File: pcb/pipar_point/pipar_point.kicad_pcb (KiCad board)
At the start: 2 copper layers, 145.3 x 110.3 mm, 118 parts, among them Q1 AO3416 N-channel MOSFET, SW1 SW_Wuerth_450301014042, SW2 CK_KMS2xxG, U1 Seeeduino Xiao nRF52840, U2 74HC595

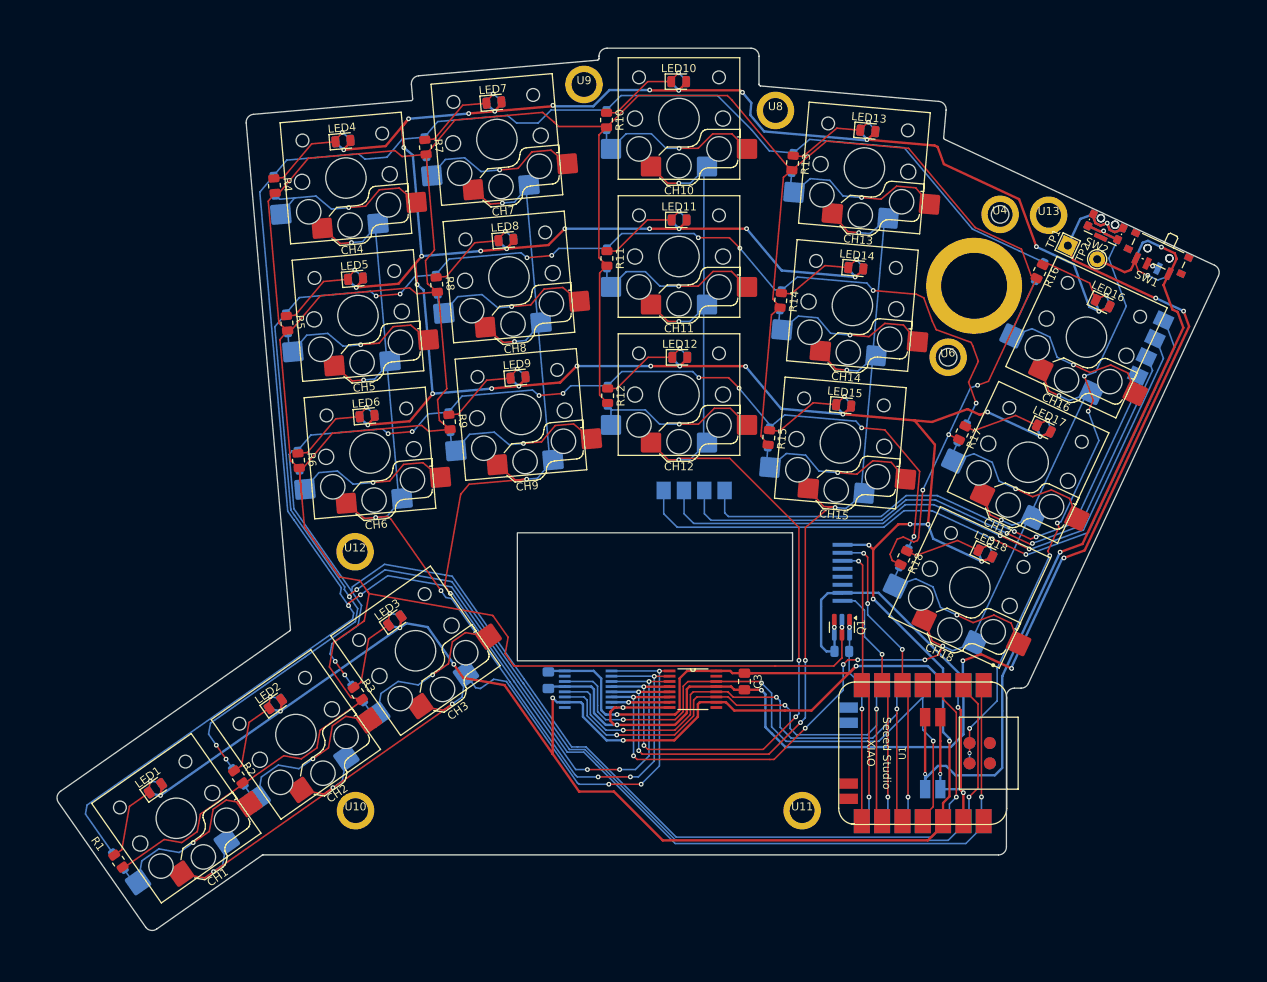
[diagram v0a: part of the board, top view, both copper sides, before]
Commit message: adds lights
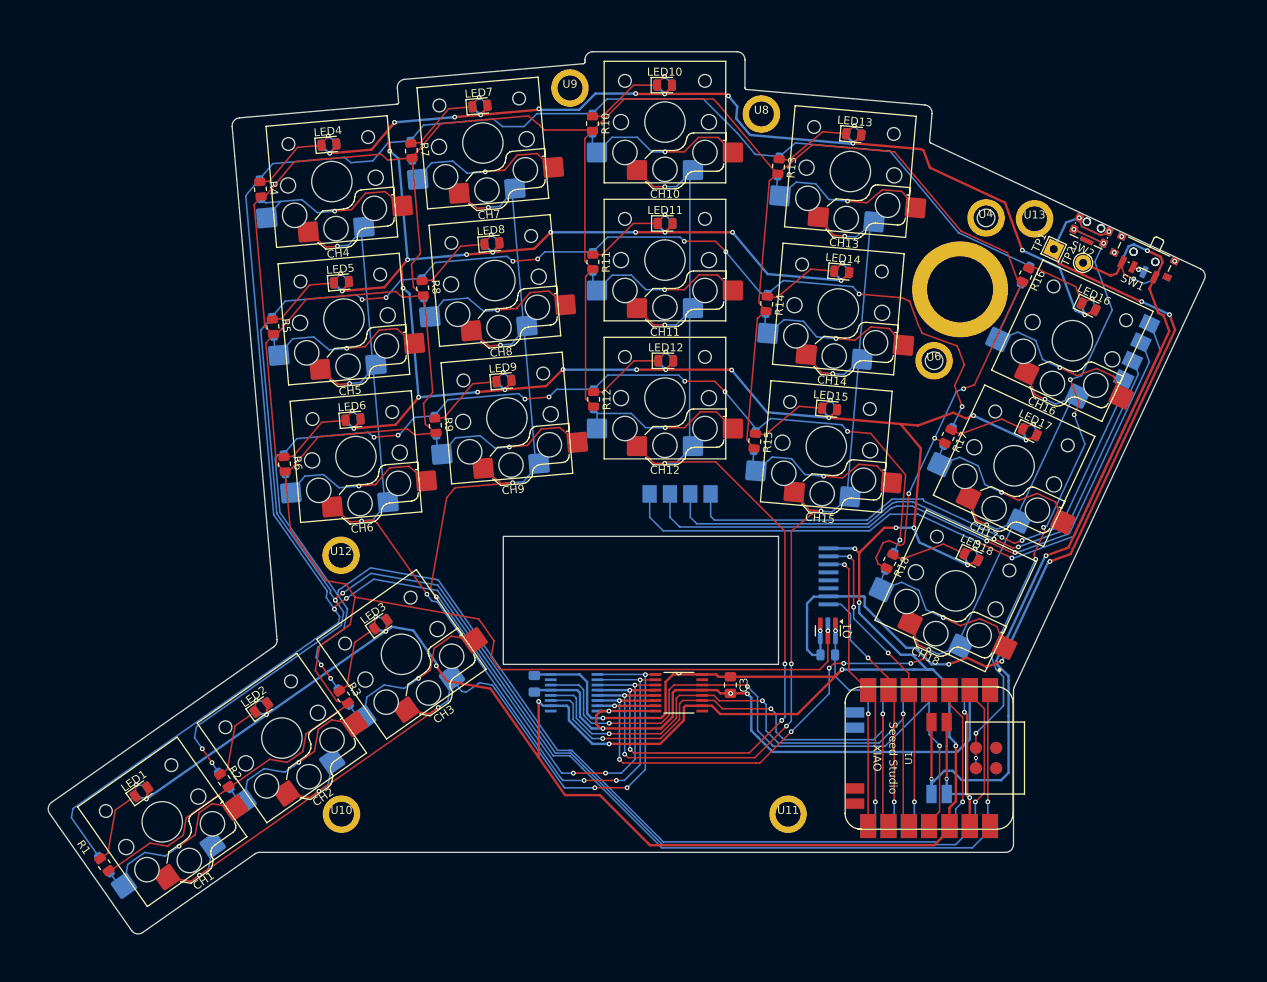
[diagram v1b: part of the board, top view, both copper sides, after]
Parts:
- removed the U1 at (195.7, 109.1) (x2)
- added U1: Seeeduino Xiao nRF52840, Seeed Studio XIAO Series Library:XIAO-nRF52840-Sense-14P-2.54-21X17.8MM, F.Cu at (196.5, 109.8)
- added U1: Seeeduino Xiao nRF52840, Seeed Studio XIAO Series Library:XIAO-nRF52840-Sense-14P-2.54-21X17.8MM, B.Cu at (196.5, 109.8)
- moved CH15 1.81 mm to (183.7, 70.8)
- moved LED9 1.81 mm to (143.4, 62.6)
- moved LED2 1.81 mm to (113.1, 103.4) (x2)
- moved D5 1.81 mm to (114.5, 55.9)
- moved R5 1.81 mm to (114.5, 55.9)
- moved D8 1.81 mm to (133.2, 51.0)
- moved R8 1.81 mm to (133.2, 51.0)
- moved LED11 1.81 mm to (163.5, 42.9) (x2)
- moved LED10 1.81 mm to (163.5, 25.6) (x2)
- moved D10 1.81 mm to (154.4, 30.4)
- moved R10 1.81 mm to (154.4, 30.4)
- moved R19 1.81 mm to (183.9, 96.9)
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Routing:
- net LEDOut: track 497.2 -> 493.5 mm
- net Earth: track 243.3 -> 239.7 mm, vias 13 -> 15
- net ROW2: track 245.2 -> 248.7 mm
- net +3V3: track 664.9 -> 668.4 mm
- net ROW1: track 292.9 -> 295.8 mm
- net ROW0: track 332.2 -> 334.8 mm
- net MOSI: track 79.8 -> 82.5 mm
- net LEDTrig: track 25.9 -> 28.5 mm
- net  SCK: track 68.6 -> 71.2 mm
- net MISO: track 72.1 -> 74.8 mm
- net TPData: track 38.8 -> 40.0 mm
- net TPCLK: track 31.1 -> 32.3 mm
- net TPRST: track 35.5 -> 36.7 mm
- net BAT+: track 99.9 -> 100.5 mm
- net Net-(U1-RST): track 81.8 -> 81.7 mm, vias 7 -> 8
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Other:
- board size 145.3 x 110.3 mm -> 144.6 x 110.3 mm
